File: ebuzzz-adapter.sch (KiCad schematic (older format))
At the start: 33 parts, among them J1 Conn_01x04, J2 Conn_01x04, J3 Conn_01x06, J4 EBUS, Q1 BC817-40, U1 CNY17-4, U2 CNY17-4, U3 LM2903, U4 LP2951-5.0_SOIC

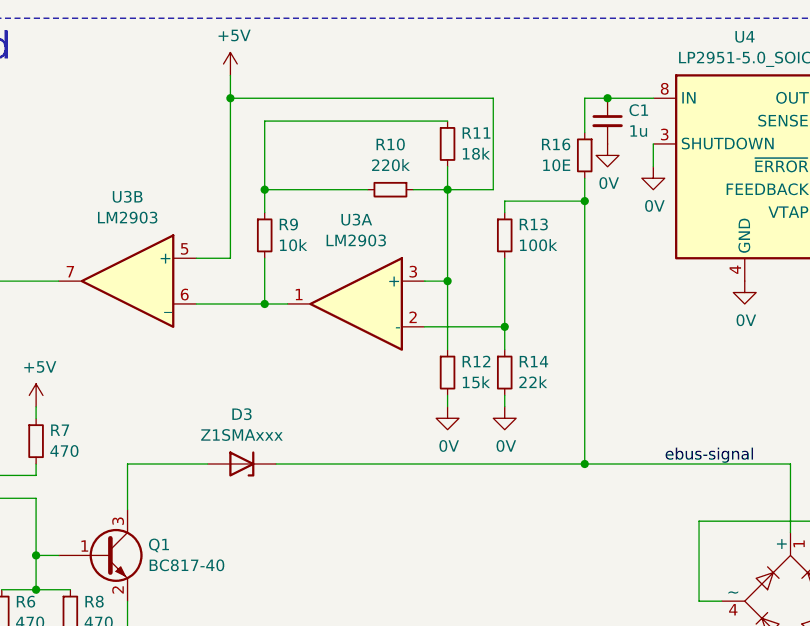
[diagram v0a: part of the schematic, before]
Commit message: Version 1 release (hardware tested)
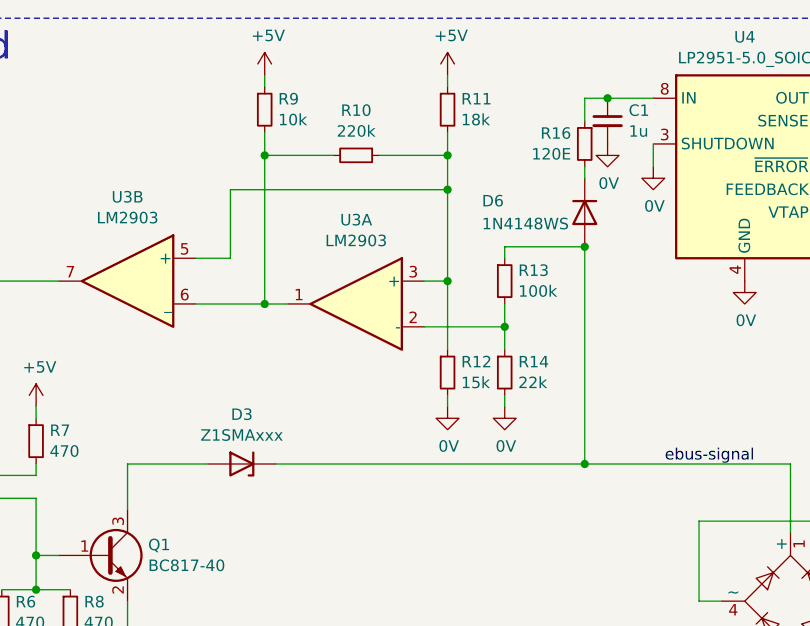
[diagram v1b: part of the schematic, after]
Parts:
- added D6: 1N4148WS, Diode_SMD:D_SOD-323, symbol Diode:1N4148WS
- D3: Farnell (none) -> 1611267
- R16: value 10E -> 120E
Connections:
- net +5V: now also R11.1, R9.1; no longer R10.1, R11.2, R12.1, U3.3 (+), U3.5 (+)
- net ebus-signal: now also D6.2 (A); no longer R16.2
- net at R9.2, U3.1, U3.6 (_): now also R10.2
- new net: R10.1, R11.2, R12.1, U3.3 (+), U3.5 (+)
- new net: D6.1 (K), R16.2
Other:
- moved on the sheet: R10, R11, R13, R16, R9
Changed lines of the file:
@@
 L Device:R_Small R11
 U 1 1 5D4C8B84
-P 7100 1250
-F 0 "R11" H 7159 1296 50  0000 L CNN
-F 1 "18k" H 7159 1205 50  0000 L CNN
-F 2 "Resistor_SMD:R_0805_2012Metric_Pad1.15x1.40mm_HandSolder" H 7100 1250 50  0001 C CNN
-F 3 "~" H 7100 1250 50  0001 C CNN
-	1    7100 1250
+P 7100 1100
+F 0 "R11" H 7159 1146 50  0000 L CNN
+F 1 "18k" H 7159 1055 50  0000 L CNN
+F 2 "Resistor_SMD:R_0805_2012Metric_Pad1.15x1.40mm_HandSolder" H 7100 1100 50  0001 C CNN
+F 3 "~" H 7100 1100 50  0001 C CNN
+	1    7100 1100
 	1    0    0    -1
 $EndComp
@@
 L Device:R_Small R13
 U 1 1 5D4C8EDF
-P 7350 1650
-F 0 "R13" H 7409 1696 50  0000 L CNN
-F 1 "100k" H 7409 1605 50  0000 L CNN
-F 2 "Resistor_SMD:R_0805_2012Metric_Pad1.15x1.40mm_HandSolder" H 7350 1650 50  0001 C CNN
-F 3 "~" H 7350 1650 50  0001 C CNN
-	1    7350 1650
+P 7350 1850
+F 0 "R13" H 7409 1896 50  0000 L CNN
+F 1 "100k" H 7409 1805 50  0000 L CNN
+F 2 "Resistor_SMD:R_0805_2012Metric_Pad1.15x1.40mm_HandSolder" H 7350 1850 50  0001 C CNN
+F 3 "~" H 7350 1850 50  0001 C CNN
+	1    7350 1850
 	1    0    0    -1
 $EndComp
@@
 L Device:R_Small R10
 U 1 1 5D4C977A
-P 6850 1450
-F 0 "R10" V 6654 1450 50  0000 C CNN
-F 1 "220k" V 6745 1450 50  0000 C CNN
-F 2 "Resistor_SMD:R_0805_2012Metric_Pad1.15x1.40mm_HandSolder" H 6850 1450 50  0001 C CNN
-F 3 "~" H 6850 1450 50  0001 C CNN
-	1    6850 1450
+P 6700 1300
+F 0 "R10" V 6504 1300 50  0000 C CNN
+F 1 "220k" V 6595 1300 50  0000 C CNN
+F 2 "Resistor_SMD:R_0805_2012Metric_Pad1.15x1.40mm_HandSolder" H 6700 1300 50  0001 C CNN
+F 3 "~" H 6700 1300 50  0001 C CNN
+	1    6700 1300
 	0    1    1    0
 $EndComp
@@
 L Device:R_Small R9
 U 1 1 5D4CA98C
-P 6300 1650
-F 0 "R9" H 6359 1696 50  0000 L CNN
-F 1 "10k" H 6359 1605 50  0000 L CNN
-F 2 "Resistor_SMD:R_0805_2012Metric_Pad1.15x1.40mm_HandSolder" H 6300 1650 50  0001 C CNN
-F 3 "~" H 6300 1650 50  0001 C CNN
-	1    6300 1650
+P 6300 1100
+F 0 "R9" H 6359 1146 50  0000 L CNN
+F 1 "10k" H 6359 1055 50  0000 L CNN
+F 2 "Resistor_SMD:R_0805_2012Metric_Pad1.15x1.40mm_HandSolder" H 6300 1100 50  0001 C CNN
+F 3 "~" H 6300 1100 50  0001 C CNN
+	1    6300 1100
 	1    0    0    -1
 $EndComp
@@
 	7350 2050 7350 2150
 Wire Wire Line
-	7350 1750 7350 2050
+	7350 1950 7350 2050
 Connection ~ 7350 2050
 Wire Wire Line
@@
 Connection ~ 7100 1850
 Wire Wire Line
-	7100 1350 7100 1450
-Wire Wire Line
-	6950 1450 7100 1450
-Connection ~ 7100 1450
-Wire Wire Line
-	7100 1450 7100 1850
-Wire Wire Line
-	7100 1150 6300 1150
-Wire Wire Line
-	6300 1150 6300 1450
-Wire Wire Line
-	6300 1450 6750 1450
-Wire Wire Line
-	6300 1450 6300 1550
-Connection ~ 6300 1450
-Wire Wire Line
-	6300 1750 6300 1950
+	7100 1200 7100 1300
+Wire Wire Line
+	6800 1300 7100 1300
+Connection ~ 7100 1300
+Wire Wire Line
+	6300 950  6300 1000
+Wire Wire Line
+	6300 1300 6600 1300
+Connection ~ 6300 1300
 Wire Wire Line
 	6300 1950 6400 1950
 Wire Wire Line
 	6000 1750 6150 1750
-Wire Wire Line
-	6150 1050 7300 1050
-Wire Wire Line
-	7300 1050 7300 1450
-Wire Wire Line
-	7300 1450 7100 1450
-Wire Wire Line
-	6150 1050 6150 1750
 Wire Wire Line
 	6000 1950 6300 1950
@@
 Wire Wire Line
 	9150 3250 9150 3000
-$Comp
-L power:+5V #PWR05
-U 1 1 5D516E86
-P 6150 950
-F 0 "#PWR05" H 6150 800 50  0001 C CNN
-F 1 "+5V" H 6165 1123 50  0000 C CNN
-F 2 "" H 6150 950 50  0001 C CNN
-F 3 "" H 6150 950 50  0001 C CNN
-	1    6150 950
-	1    0    0    -1
-$EndComp
-Wire Wire Line
-	6150 950  6150 1050
-Connection ~ 6150 1050
 $Comp
 L power:+5V #PWR01
@@
 	8600 2650 7700 2650
 Wire Wire Line
-	7700 2650 7700 1500
-Wire Wire Line
-	7700 1500 7350 1500
-Wire Wire Line
-	7350 1500 7350 1550
+	7700 2650 7700 1700
+Wire Wire Line
+	7700 1700 7350 1700
+Wire Wire Line
+	7350 1700 7350 1750
 $Comp
 L power:0V #PWR010
@@
 	8000 1250 8000 1350
 Wire Wire Line
-	7700 1050 7700 1200
-Connection ~ 7700 1500
+	7700 1050 7700 1150
 Wire Wire Line
 	7700 1050 7800 1050
@@
 F 2 "Diode_SMD:D_SMA" H 6200 2475 50  0001 C CNN
 F 3 "https://diotec.com/tl_files/diotec/files/pdf/datasheets/z1sma1.pdf" H 6200 2650 50  0001 C CNN
+F 4 "1611267" H 6200 2650 50  0001 C CNN "Farnell"
 	1    6200 2650
 	-1   0    0    1
@@
 L Device:R_Small R16
 U 1 1 5D77CA1D
-P 7700 1300
-F 0 "R16" H 7759 1346 50  0000 L CNN
-F 1 "10E" H 7759 1255 50  0000 L CNN
-F 2 "Resistor_SMD:R_0805_2012Metric_Pad1.15x1.40mm_HandSolder" H 7700 1300 50  0001 C CNN
-F 3 "~" H 7700 1300 50  0001 C CNN
-	1    7700 1300
+P 7700 1250
+F 0 "R16" H 7759 1296 50  0000 L CNN
+F 1 "120E" H 7759 1205 50  0000 L CNN
+F 2 "Resistor_SMD:R_0805_2012Metric_Pad1.15x1.40mm_HandSolder" H 7700 1250 50  0001 C CNN
+F 3 "~" H 7700 1250 50  0001 C CNN
+	1    7700 1250
 	-1   0    0    -1
 $EndComp
-Wire Wire Line
-	7700 1400 7700 1500
-$Comp
-L power:0V #PWR?
+$Comp
+L power:0V #PWR0101
 U 1 1 5D521163
 P 5700 3450
-F 0 "#PWR?" H 5700 3200 50  0001 C CNN
+F 0 "#PWR0101" H 5700 3200 50  0001 C CNN
 F 1 "0V" H 5705 3277 50  0000 C CNN
 F 2 "" H 5700 3450 50  0001 C CNN
@@
 	1    0    0    -1
 $EndComp
+Wire Wire Line
+	7100 950  7100 1000
+$Comp
+L power:+5V #PWR04
+U 1 1 5D5B09A3
+P 6300 950
+F 0 "#PWR04" H 6300 800 50  0001 C CNN
+F 1 "+5V" H 6315 1123 50  0000 C CNN
+F 2 "" H 6300 950 50  0001 C CNN
+F 3 "" H 6300 950 50  0001 C CNN
+	1    6300 950
+	1    0    0    -1
+$EndComp
+Wire Wire Line
+	6150 1450 6150 1750
+Wire Wire Line
+	7100 1450 7100 1850
+Connection ~ 7100 1450
+Wire Wire Line
+	7100 1300 7100 1450
+Wire Wire Line
+	7100 1450 6150 1450
+$Comp
+L power:+5V #PWR05
+U 1 1 5D516E86
+P 7100 950
+F 0 "#PWR05" H 7100 800 50  0001 C CNN
+F 1 "+5V" H 7115 1123 50  0000 C CNN
+F 2 "" H 7100 950 50  0001 C CNN
+F 3 "" H 7100 950 50  0001 C CNN
+	1    7100 950
+	1    0    0    -1
+$EndComp
+Wire Wire Line
+	6300 1200 6300 1300
+Wire Wire Line
+	6300 1300 6300 1950
+$Comp
+L Diode:1N4148WS D6
+U 1 1 5DACF05D
+P 7700 1550
+F 0 "D6" V 7650 1100 50  0000 L CNN
+F 1 "1N4148WS" V 7750 1100 50  0000 L CNN
+F 2 "Diode_SMD:D_SOD-323" H 7700 1375 50  0001 C CNN
+F 3 "https://www.vishay.com/docs/85751/1n4148ws.pdf" H 7700 1550 50  0001 C CNN
+F 4 "2675148" V 7700 1550 50  0001 C CNN "Farnell"
+	1    7700 1550
+	0    1    1    0
+$EndComp
+Connection ~ 7700 1700
+Wire Wire Line
+	7700 1350 7700 1400
 $EndSCHEMATC
